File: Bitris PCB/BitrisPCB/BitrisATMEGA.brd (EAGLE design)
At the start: 49.2 x 50.8 mm, 27 parts, among them IC1 ATMEGA328-20P, IC2 4511N, X1 Boton, X2 Sonido, X3 Alimentacion, X4 Monedas

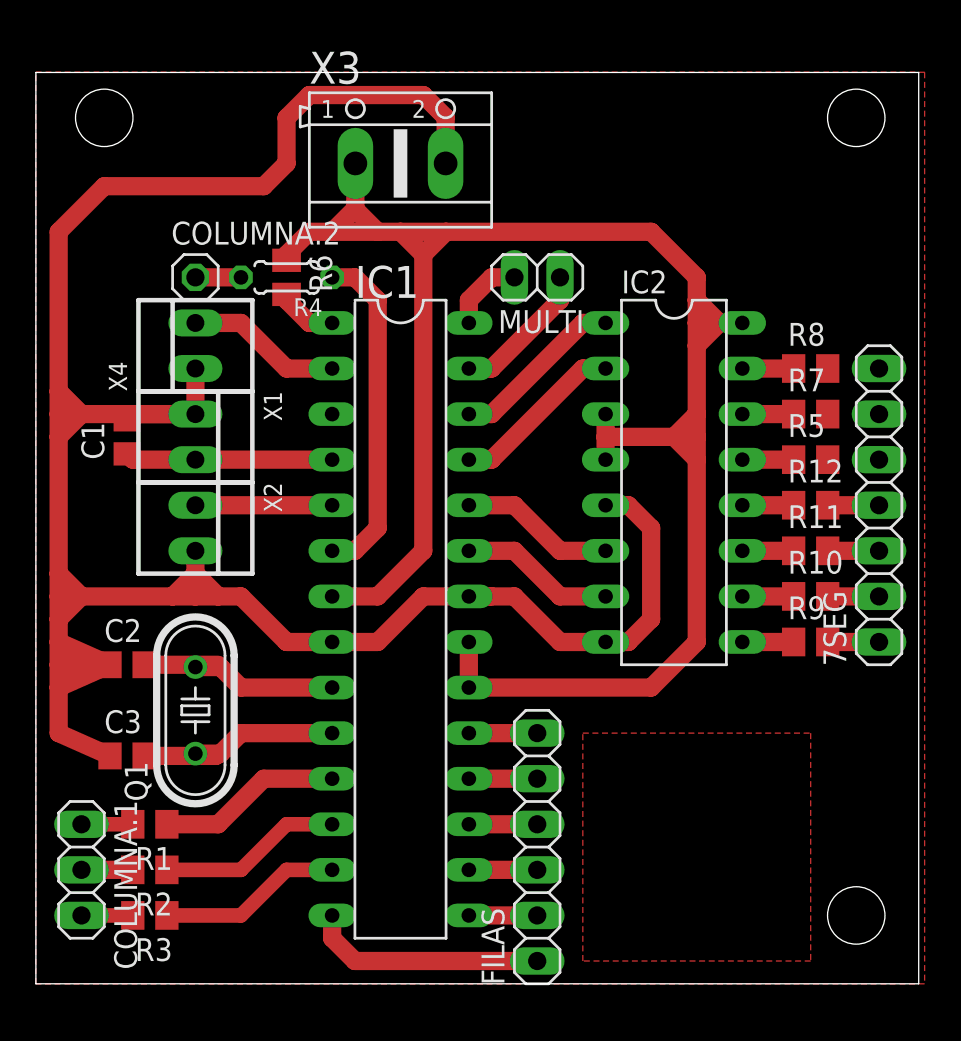
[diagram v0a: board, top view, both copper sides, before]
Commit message: Ajuste SCH
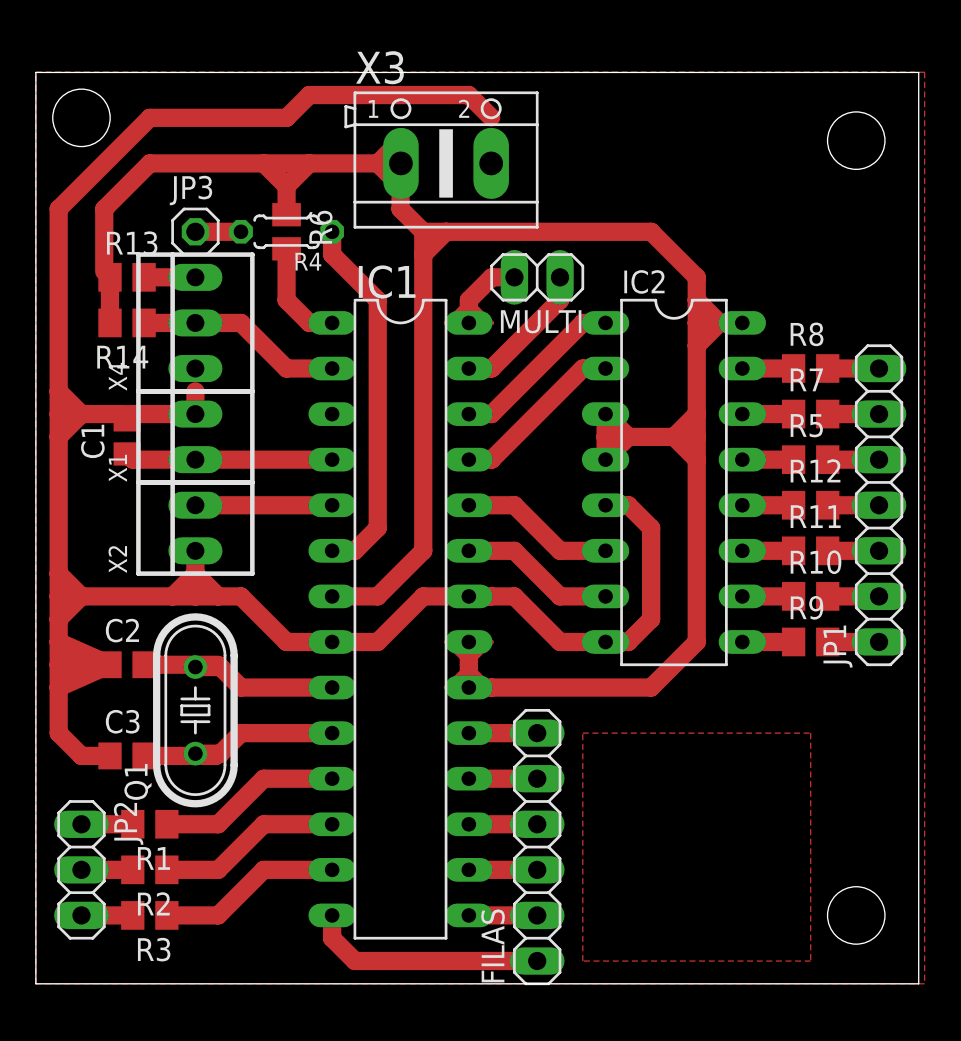
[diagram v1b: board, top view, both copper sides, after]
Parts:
- removed COLUMNA.2: (no value), pinhead:1X01
- added JP3: (no value), pinhead:1X01
- added R13, R14: (no value), rcl:M0805
- R1, R10, R11, R12, R2, R3, R4, R5, R7, R8, R9: value 220 -> (none)
- R6: value 10k -> (none)
- X4: value Monedas -> MONEDA; device con-molex:22-23-2021 -> con-molex:22-23-2031
- moved R4 2.54 mm to (49.5, 50.8)
- moved R6 2.54 mm to (49.5, 50.8)
- moved X3 2.54 mm to (58.4, 54.6)
- moved X4 1.27 mm to (44.5, 45.7)
- turned X1 to 90 degrees
- turned X2 to 90 degrees
- renumbered 7SEG to JP1, COLUMNA.1 to JP2
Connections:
- new net N$44: R13.2, X4.3
- net GND: now also X1.2, X2.1; no longer X1.1, X2.2
- net N$30: now also R14.1
- net N$32: now also X2.2; no longer X2.1
- net N$33: now also X1.1; no longer X1.2
- net N$4: now also JP3.1; no longer COLUMNA.2.1
- net VCC: now also R13.1, R14.2
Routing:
- net VCC: track 111.1 -> 144.4 mm
- net N$16: track 4.34 -> 10.5 mm
- net GND: track 143.0 -> 137.9 mm
- net N$44: track 0.00 -> 2.86 mm
- net N$41: track 0.00 -> 2.86 mm
- net N$40: track 0.00 -> 2.86 mm
- net N$39: track 0.00 -> 2.86 mm
- net N$30: track 8.67 -> 11.5 mm
- net N$34: track 3.39 -> 5.93 mm
- net N$17: track 18.8 -> 20.6 mm
